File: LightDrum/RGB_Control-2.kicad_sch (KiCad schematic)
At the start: 25 parts, among them Q12 PMXB43UNEZ, Q13 PMXB43UNEZ, Q14 PMXB43UNEZ, Q15 PMXB43UNEZ, Q16 PMXB43UNEZ, Q17 PMXB43UNEZ, Q18 PMXB43UNEZ, Q19 PMXB43UNEZ, U10 PCA9634_TSSOP20

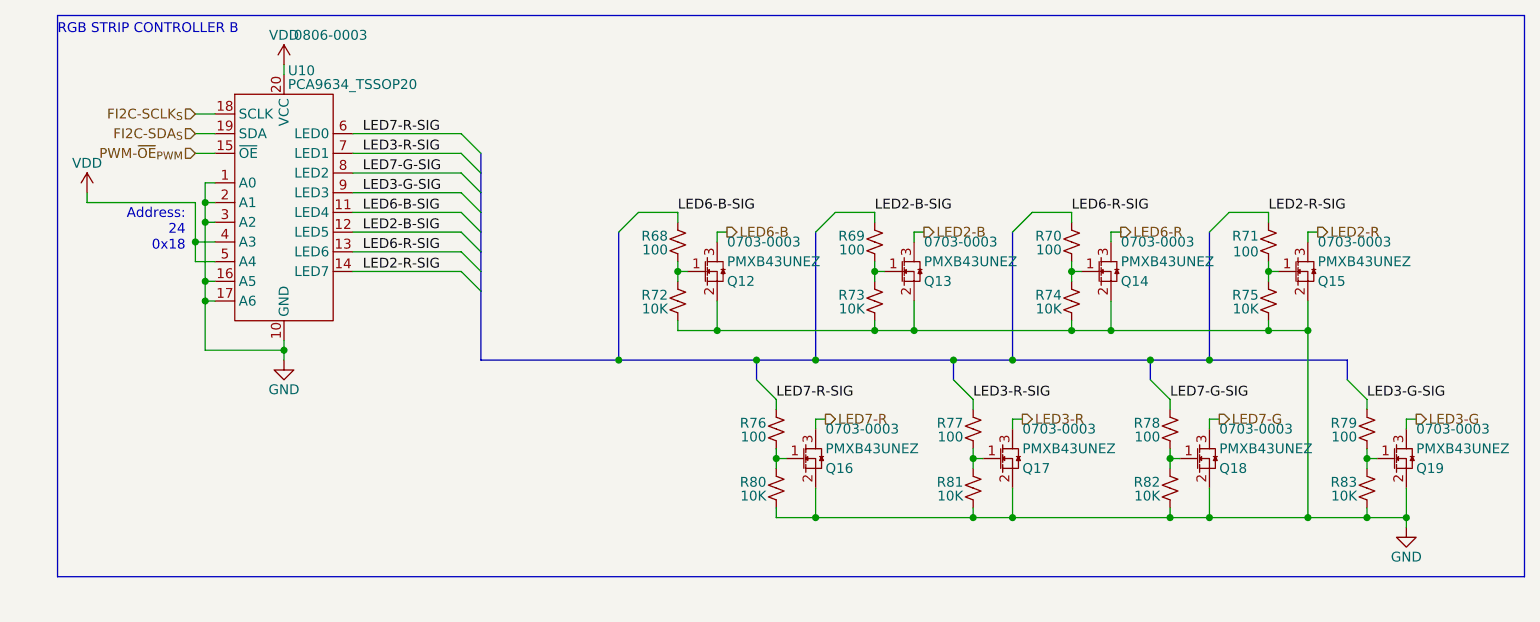
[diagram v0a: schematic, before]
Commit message: Minor fixes and cleanup - REV11
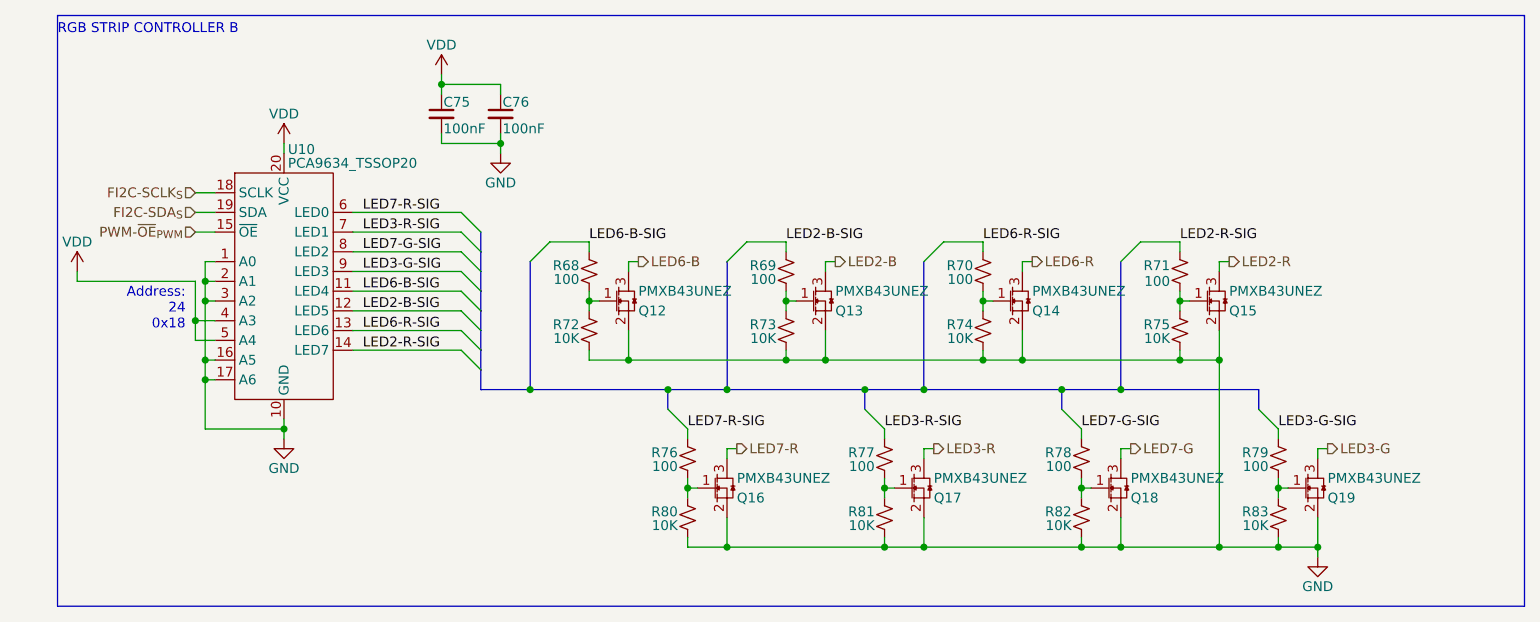
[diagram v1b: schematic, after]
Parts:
- added C75, C76: 100nF, Capacitor_SMD:C_0402_1005Metric, symbol Daxxn_Device:C
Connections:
- net GND: now also C75.2, C76.2
- net VDD: now also C75.1, C76.1
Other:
- moved on the sheet: Q12, Q13, Q14, Q15, Q16, Q17, Q18, Q19, R68, R69, R70, R71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
